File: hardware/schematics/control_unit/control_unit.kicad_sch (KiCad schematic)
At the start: 14 parts, among them J1 Screw_Terminal_01x12, J2 Screw_Terminal_01x08, J3 Screw_Terminal_01x08, J4 AudioJack4, J5 Screw_Terminal_01x08, J6 6P6C, J7 Conn_01x03_Pin, J8 Conn_01x03_Pin

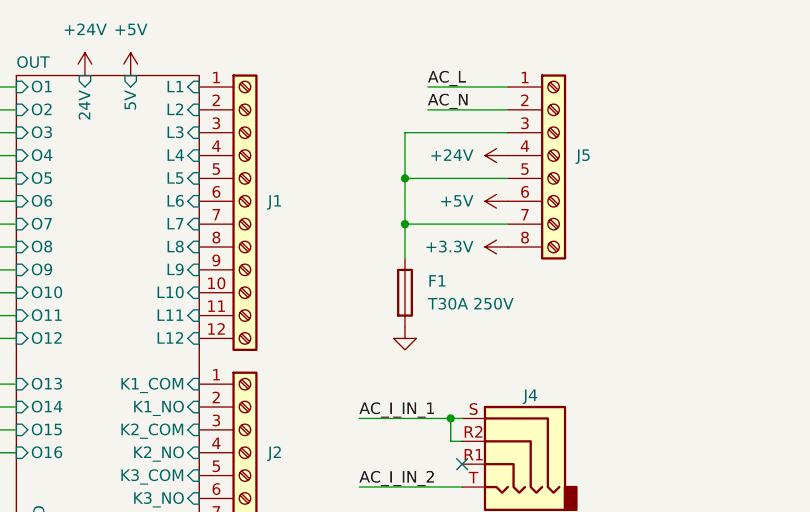
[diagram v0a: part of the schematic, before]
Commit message: !feat: control_unit first PCB release.
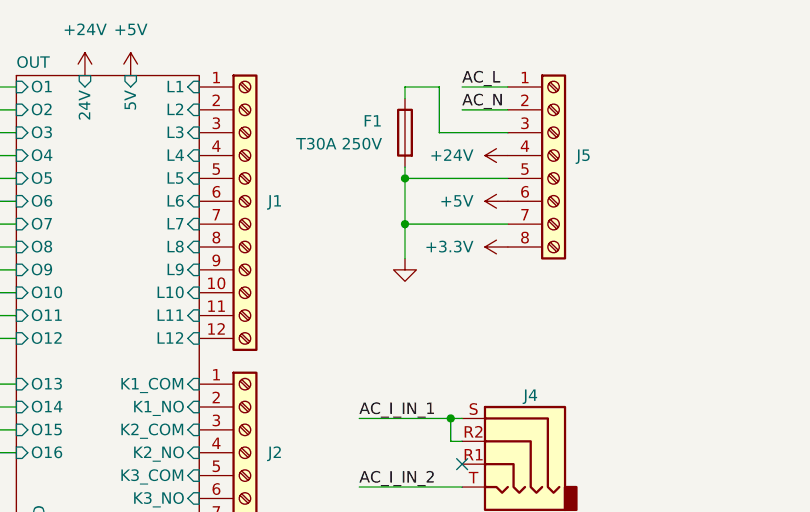
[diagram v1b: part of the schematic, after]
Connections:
- net GND: now also J5.5 (Pin_5), J5.7 (Pin_7)
- net at F1.1, J5.3 (Pin_3): no longer J5.5 (Pin_5), J5.7 (Pin_7)
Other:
- moved on the sheet: F1
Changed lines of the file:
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@@
+	)
+	(junction
+		(at 165.1 36.83)
+		(diameter 0)
+		(color 0 0 0 0)
 	)
 	(junction
@@
 	)
 	(junction
-		(at 165.1 36.83)
-		(diameter 0)
-		(color 0 0 0 0)
-	)
-	(junction
 		(at 119.38 121.92)
 		(diameter 0)
@@
 	(wire
 		(pts
+			(xy 168.91 26.67) (xy 165.1 26.67)
+		)
+		(stroke
+			(width 0)
+			(type default)
+		)
+	)
+	(wire
+		(pts
 			(xy 165.1 41.91) (xy 176.53 41.91)
 		)
@@
 	(wire
 		(pts
+			(xy 165.1 26.67) (xy 165.1 27.94)
+		)
+		(stroke
+			(width 0)
+			(type default)
+		)
+	)
+	(wire
+		(pts
 			(xy 148.59 91.44) (xy 172.72 91.44)
 		)
@@
 	(wire
 		(pts
-			(xy 176.53 31.75) (xy 165.1 31.75)
-		)
-		(stroke
-			(width 0)
-			(type default)
-		)
-	)
-	(wire
-		(pts
 			(xy 53.34 44.45) (xy 63.5 44.45)
 		)
@@
 	(wire
 		(pts
+			(xy 168.91 31.75) (xy 168.91 26.67)
+		)
+		(stroke
+			(width 0)
+			(type default)
+		)
+	)
+	(wire
+		(pts
 			(xy 148.59 101.6) (xy 156.21 101.6)
 		)
@@
 	(wire
 		(pts
+			(xy 165.1 35.56) (xy 165.1 36.83)
+		)
+		(stroke
+			(width 0)
+			(type default)
+		)
+	)
+	(wire
+		(pts
 			(xy 177.8 124.46) (xy 182.88 124.46)
 		)
@@
 	(wire
 		(pts
-			(xy 167.64 26.67) (xy 176.53 26.67)
+			(xy 171.45 26.67) (xy 176.53 26.67)
 		)
 		(stroke
@@
 	(wire
 		(pts
-			(xy 167.64 29.21) (xy 176.53 29.21)
+			(xy 171.45 29.21) (xy 176.53 29.21)
 		)
 		(stroke
@@
 	(wire
 		(pts
+			(xy 176.53 31.75) (xy 168.91 31.75)
+		)
+		(stroke
+			(width 0)
+			(type default)
+		)
+	)
+	(wire
+		(pts
 			(xy 111.76 64.77) (xy 121.92 64.77)
 		)
@@
 	(wire
 		(pts
-			(xy 165.1 31.75) (xy 165.1 36.83)
-		)
-		(stroke
-			(width 0)
-			(type default)
-		)
-	)
-	(wire
-		(pts
 			(xy 165.1 41.91) (xy 165.1 45.72)
 		)
@@
 	)
 	(label "AC_N"
-		(at 167.64 29.21 0)
+		(at 171.45 29.21 0)
 		(fields_autoplaced yes)
 		(effects
@@
 	)
 	(label "AC_L"
-		(at 167.64 26.67 0)
+		(at 171.45 26.67 0)
 		(fields_autoplaced yes)
 		(effects
@@
 	(symbol
 		(lib_id "Device:Fuse")
-		(at 165.1 49.53 0)
+		(at 165.1 31.75 0)
+		(mirror y)
 		(unit 1)
 		(exclude_from_sim no)
@@
 		(on_board yes)
 		(dnp no)
-		(fields_autoplaced yes)
 		(property "Reference" "F1"
-			(at 167.64 48.2599 0)
+			(at 162.56 30.4799 0)
 			(effects
 				(font
@@
 		)
 		(property "Value" "T30A 250V"
-			(at 167.64 50.7999 0)
+			(at 162.56 33.0199 0)
 			(effects
 				(font
@@
 		)
 		(property "Footprint" "Fuse:Fuseholder_Clip-6.3x32mm_Littelfuse_102_Inline_P34.21x7.62mm_D2.54mm_Horizontal"
-			(at 163.322 49.53 90)
+			(at 166.878 31.75 90)
 			(effects
 				(font
@@
 		)
 		(property "Datasheet" "~"
-			(at 165.1 49.53 0)
+			(at 165.1 31.75 0)
 			(effects
 				(font
@@
 		)
 		(property "Description" "Fuse"
-			(at 165.1 49.53 0)
+			(at 165.1 31.75 0)
 			(effects
 				(font
@@
 	(symbol
 		(lib_id "power:GND")
-		(at 165.1 53.34 0)
+		(at 165.1 45.72 0)
 		(unit 1)
 		(exclude_from_sim no)
@@
 		(fields_autoplaced yes)
 		(property "Reference" "#PWR019"
-			(at 165.1 59.69 0)
+			(at 165.1 52.07 0)
 			(effects
 				(font
@@
 		)
 		(property "Value" "GND"
-			(at 165.1 58.42 0)
+			(at 165.1 50.8 0)
 			(effects
 				(font
@@
 		)
 		(property "Footprint" ""
-			(at 165.1 53.34 0)
+			(at 165.1 45.72 0)
 			(effects
 				(font
@@
 		)
 		(property "Datasheet" ""
-			(at 165.1 53.34 0)
+			(at 165.1 45.72 0)
 			(effects
 				(font
@@
 		)
 		(property "Description" "Power symbol creates a global label with name \"GND\" , ground"
-			(at 165.1 53.34 0)
-			(effects
-				(font
+			(at 165.1 45.72 0)
+			(effects
+				(font
